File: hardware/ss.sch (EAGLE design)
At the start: 76 parts, among them IC1 DS3231, Q1 BSS138, Q3 si2305cd, Q4 si2305cd, Q5 8MHz, Q6 si2305cd, U1 SPX5205 3v3, U17 AVR_SPI_PRG_6PTH, U2 CN3083, U3 SPX5205 3v3, U5 ATMEGA328, U6 microSD Socket, X1 USBSMD

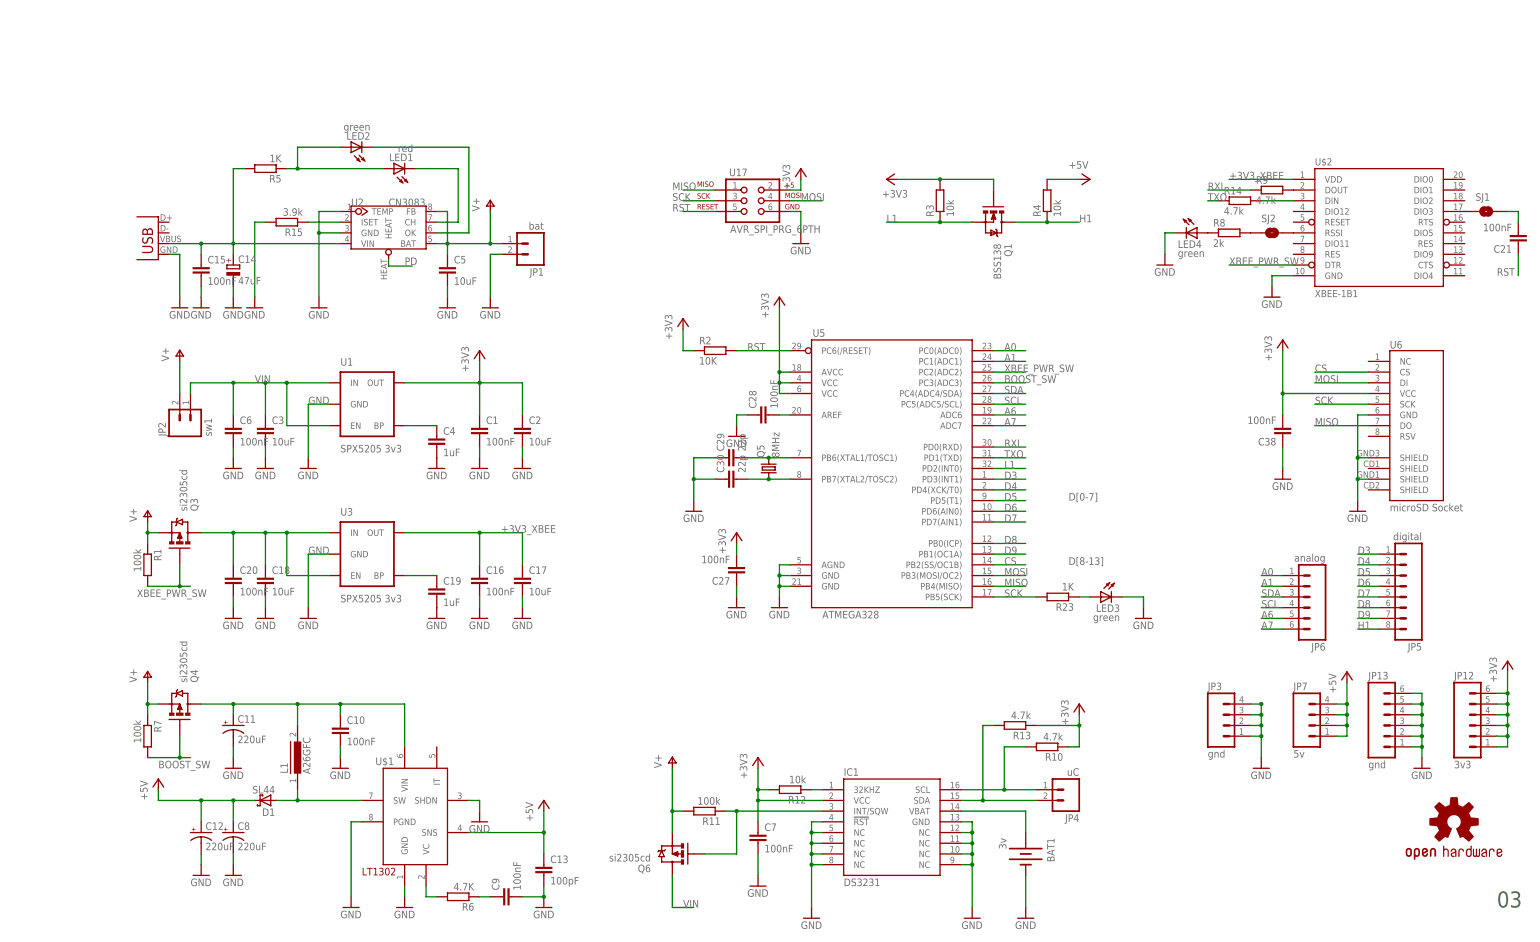
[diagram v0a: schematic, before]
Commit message: latest
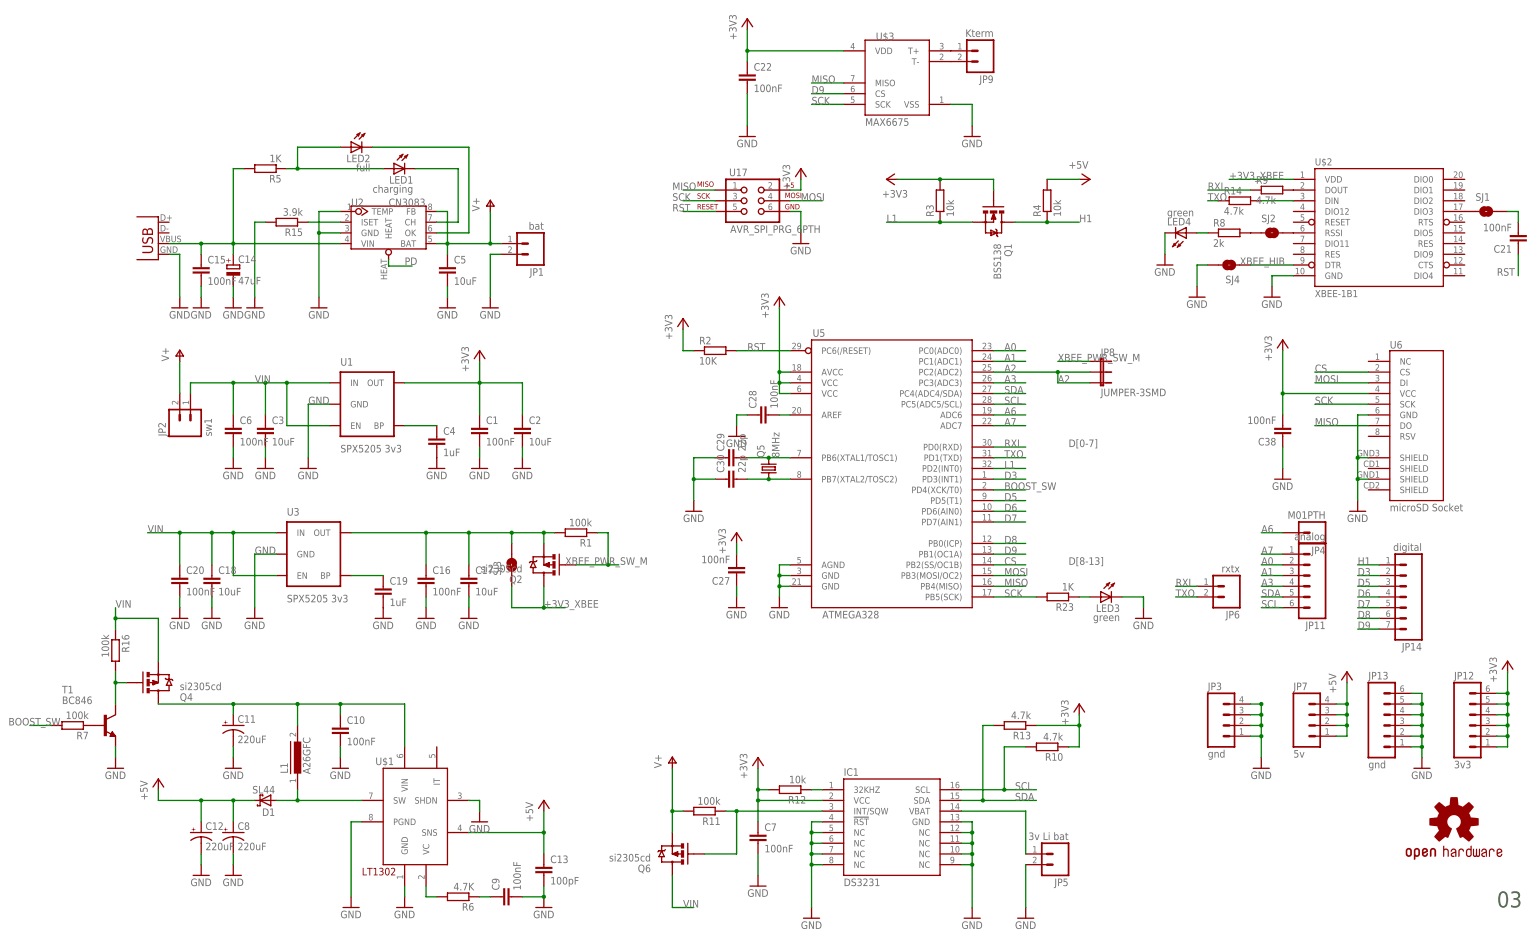
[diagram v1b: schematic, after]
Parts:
- removed BAT1: 3v, SparkFun:BATTERY12MM
- removed Q3: si2305cd, Simplex-DiscreteSemi:MOSFET-PCHANNELSMD_POWER
- added C22: 100nF, rcl:C-EUC0805
- added JP11: analog, SparkFun:M06SIP
- added JP14: digital, SparkFun-Connectors:M07
- added JP8: JUMPER-3SMD, SparkFun-Passives:JUMPER-3SMD
- added JP9: Kterm, SparkFun:M02PTH
- added Q2: si2305cd, Simplex-DiscreteSemi:MOSFET-PCHANNELSMD_POWER
- added R16: 100k, rcl:R-EU_R0805W
- added SJ3, SJ4: SOLDERJUMPERTRACE, SparkFun-Passives:SOLDERJUMPERTRACE
- added T1: BC846, transistor:BC846
- added U$3: MAX6675, SparkFun-AnalogIC:MAX6675
- JP4: value uC -> M01PTH; device SparkFun:M02PTH -> SparkFun-Connectors:M01PTH
- JP5: value digital -> 3v Li bat; device SparkFun-Connectors:M081X08 -> SparkFun:M02PTH
- JP6: value analog -> rxtx; device SparkFun-Connectors:M06SIP -> SparkFun:M02PTH
- LED1: value red -> charging; device SparkFun:LED0603 -> led:LEDCHIP-LED0805
- LED2: value green -> full; device SparkFun:LED0603 -> led:LEDCHIP-LED0805
- LED4: device SparkFun:LED0603 -> led:LEDCHIP-LED0805
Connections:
- removed net D4: JP5.2, U5.PD4(XCK/T0)
- removed net N$4: IC1.SDA, JP4.2, R13.2
- removed net N$6: IC1.SCL, JP4.1, R10.2
- removed net XBEE_IN: C18.1, C20.1, Q3.D, U3.EN, U3.IN
- removed net XBEE_PWR_SW: Q3.G, R1.2, U$2.DTR, U5.PC2(ADC2)
- new net A2: JP8.2, JP8.3, U5.PC2(ADC2)
- new net A3: JP11.4, U5.PC3(ADC3)
- new net N$100: C16.1, C17.1, Q2.S, R1.2, SJ3.2, U3.OUT
- new net N$26: R7.1, T1.B
- new net N$27: Q4.G, R16.2, T1.C
- new net N$29: JP9.1, U$3.T+
- new net N$30: JP9.2, U$3.T-
- new net XBEE_HIB: SJ4.1, U$2.DTR
- new net XBEE_PWR_SW_M: JP8.1, Q2.G, R1.1
- net +3V3: now also C22.1, U$3.VDD
- net +3V3_XBEE: now also Q2.D, SJ3.1; no longer C16.1, C17.1, U3.OUT
- net A0: now also JP11.2; no longer JP6.1
- net A1: now also JP11.3; no longer JP6.2
- net A6: now also JP4.1; no longer JP6.5
- net A7: now also JP11.1; no longer JP6.6
- net BOOST_SW: now also U5.PD4(XCK/T0); no longer Q4.G, U5.PC3(ADC3)
- net D3: now also JP14.2; no longer JP5.1
- net D5: now also JP14.3; no longer JP5.3
- net D6: now also JP14.4; no longer JP5.4
- net D7: now also JP14.5; no longer JP5.5
- net D8: now also JP14.6; no longer JP5.6
- net D9: now also JP14.7, U$3.CS; no longer JP5.7
- net GND: now also C22.2, JP5.2, SJ4.2, T1.E, U$3.VSS; no longer BAT1.-
- net H1: now also JP14.1; no longer JP5.8
- net MISO: now also U$3.MISO
- net N$10: now also JP5.1; no longer BAT1.+
- net RXI: now also JP6.1
- net SCK: now also U$3.SCK
- net SCL: now also IC1.SCL, JP11.6, R10.2; no longer JP6.4
- net SDA: now also IC1.SDA, JP11.5, R13.2; no longer JP6.3
- net TXO: now also JP6.2
- net V+: no longer Q3.S, Q4.S, R1.1, R7.1
- net VIN: now also C18.1, C20.1, Q4.S, R16.1, U3.EN, U3.IN
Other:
- moved on the sheet: C16, C17, C18, C19, C20, LED1, LED2, LED4, Q4, R1, R7, U3
